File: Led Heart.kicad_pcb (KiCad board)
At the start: 2 copper layers, 32.2 x 28.7 mm, 38 parts, among them J1 Conn_01x03_Female, J2 Conn_01x02_Female, SW1 SW_DIP_x01, U1 STM32L031G6U6

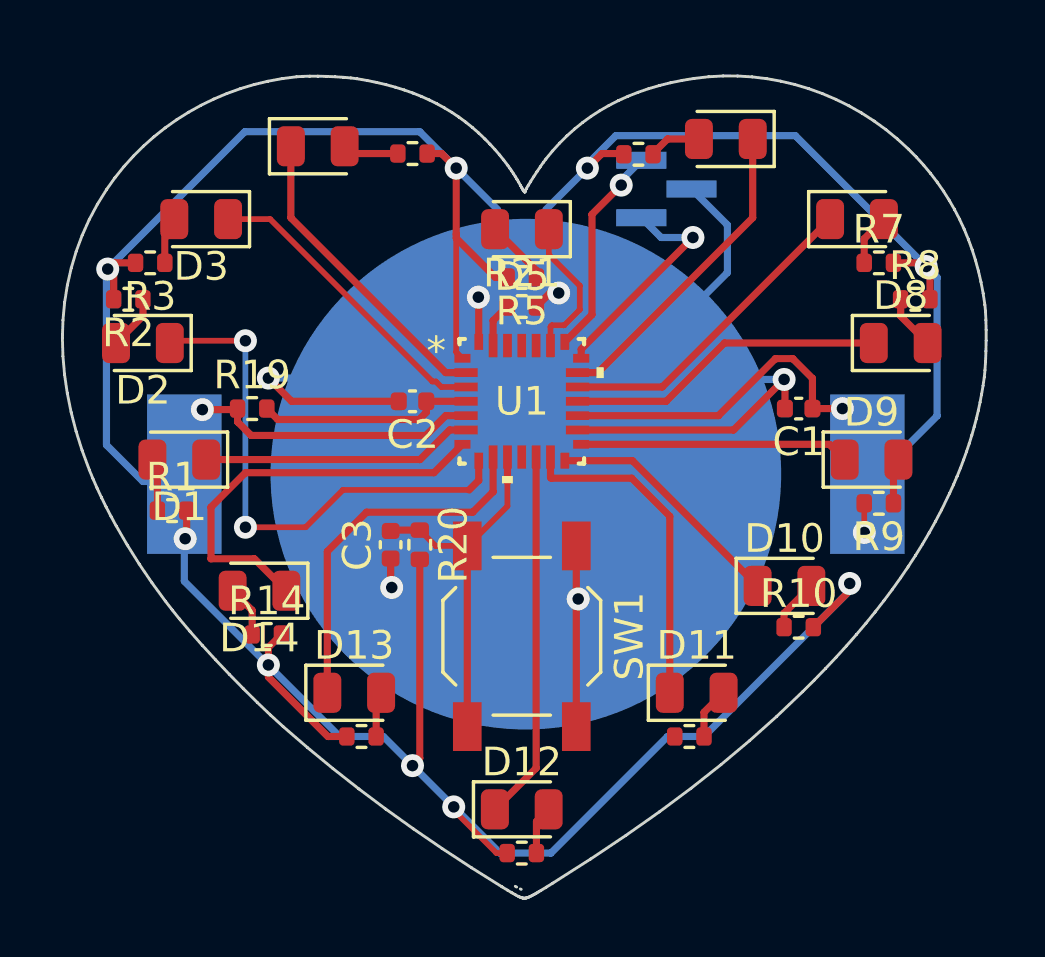
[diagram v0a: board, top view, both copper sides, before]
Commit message: Usuniety projekt emila dodany przypadkiem i ostatnie chyba poprawki
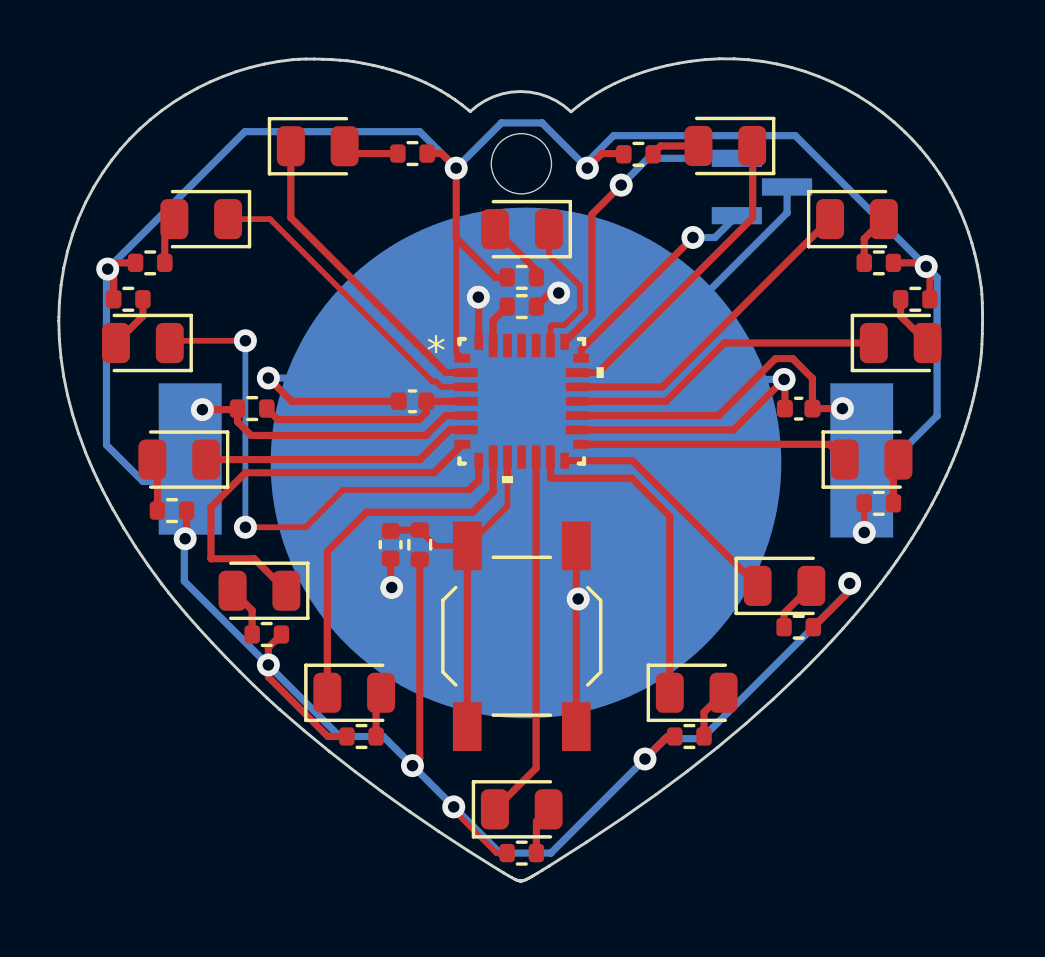
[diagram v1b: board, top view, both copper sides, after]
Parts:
- added REF**: MountingHole_2.1mm, MountingHole:MountingHole_2.1mm, F.Cu at (106.9, 84.4)
- J2: footprint Battery:BatteryHolder_MPD_BC2003_1x2032 -> SamacSys_Parts:BatteryHolder_MPD_BC2003_1x2032
- moved J1 3.33 mm to (115.3, 85.2)
- moved J2 0.39 mm to (107.1, 94.9)
- moved D6 0.24 mm to (114.0, 83.8)
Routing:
- net Net-(J1-Pad3): track 7.43 -> 10.7 mm
- net +3V0: track 143.3 -> 146.5 mm, vias 12 -> 13
- net GND: track 65.5 -> 67.4 mm
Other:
- outline, holes or cut-outs redrawn

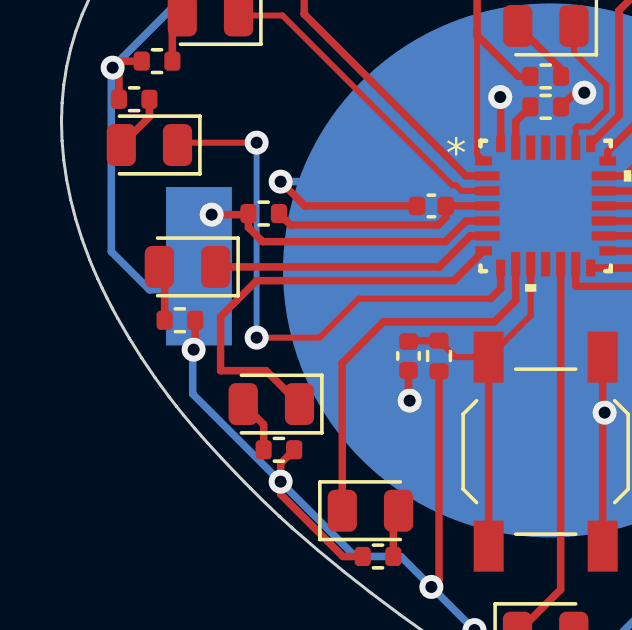
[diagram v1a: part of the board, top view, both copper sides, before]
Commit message: okkk
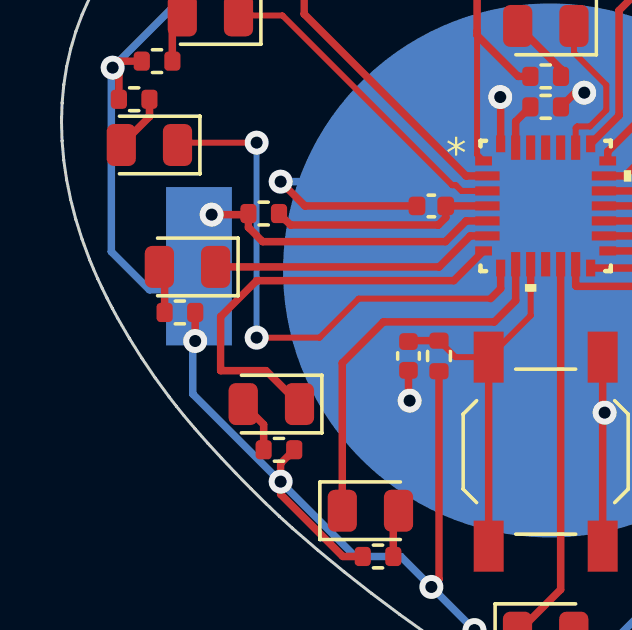
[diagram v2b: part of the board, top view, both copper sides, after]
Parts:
- moved R1 0.26 mm to (94.7, 96.3)
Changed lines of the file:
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@@
   )
   (footprint "Resistor_SMD:R_0402_1005Metric" (layer "F.Cu")
-    (at 94.742 96.52)
+    (at 94.742 96.26)
     (descr "Resistor SMD 0402 (1005 Metric), square (rectangular) end terminal, IPC_7351 nominal, (Body size source: IPC-SM-782 page 72, https://www.pcb-3d.com/wordpress/wp-content/uploads/ipc-sm-782a_amendment_1_and_2.pdf), generated with kicad-footprint-generator")
     (tags "resistor")
@@
   (gr_line (start 98.953544 80.800999) (end 99.161225 80.786298) (layer "Edge.Cuts") (width 0.1))
   (segment (start 94.232 94.9155) (end 94.0585 94.742) (width 0.25) (layer "F.Cu") (net 1))
-  (segment (start 94.232 96.52) (end 94.232 94.9155) (width 0.25) (layer "F.Cu") (net 1))
+  (segment (start 94.232 96.26) (end 94.232 94.9155) (width 0.25) (layer "F.Cu") (net 1))
   (segment (start 93.728 89.7385) (end 92.7885 90.678) (width 0.25) (layer "F.Cu") (net 2))
   (segment (start 93.728 89.154) (end 93.728 89.7385) (width 0.25) (layer "F.Cu") (net 2))
@@
   (segment (start 104.562 106.968479) (end 106.051521 108.458) (width 0.2) (layer "F.Cu") (net 16))
   (segment (start 109.728 84.074) (end 109.22 84.582) (width 0.25) (layer "F.Cu") (net 16))
+  (segment (start 95.252 97.212) (end 95.252 96.26) (width 0.25) (layer "F.Cu") (net 16))
   (segment (start 103.634 84.074) (end 104.14 84.074) (width 0.25) (layer "F.Cu") (net 16))
   (segment (start 96.99 93) (end 97.026 92.964) (width 0.25) (layer "F.Cu") (net 16))
@@
   (segment (start 97.5 93.9) (end 97.026 93.426) (width 0.25) (layer "F.Cu") (net 16))
   (segment (start 110.488 84.074) (end 109.728 84.074) (width 0.25) (layer "F.Cu") (net 16))
-  (segment (start 95.252 97.448) (end 95.2 97.5) (width 0.25) (layer "F.Cu") (net 16))
   (segment (start 104.9909 93.209999) (end 104.282102 93.209999) (width 0.25) (layer "F.Cu") (net 16))
   (segment (start 104.648 86.888) (end 104.648 90.9941) (width 0.2) (layer "F.Cu") (net 16))
@@
   (segment (start 118.872 97.282) (end 118.872 96.268) (width 0.2) (layer "F.Cu") (net 16))
   (segment (start 104.648 86.888) (end 104.648 87.023834) (width 0.25) (layer "F.Cu") (net 16))
-  (segment (start 95.252 96.52) (end 95.252 97.448) (width 0.25) (layer "F.Cu") (net 16))
   (segment (start 98.1 101.9) (end 98.1 101.292) (width 0.25) (layer "F.Cu") (net 16))
   (segment (start 92.716 87.884) (end 92.5 88.1) (width 0.25) (layer "F.Cu") (net 16))
@@
   (via (at 118.11 92.964) (size 0.8) (drill 0.4) (layers "F.Cu" "B.Cu") (net 16))
   (via (at 104.648 84.582) (size 0.8) (drill 0.4) (layers "F.Cu" "B.Cu") (net 16))
-  (via (at 95.2 97.5) (size 0.8) (drill 0.4) (layers "F.Cu" "B.Cu") (net 16))
+  (via (at 95.252 97.212) (size 0.8) (drill 0.4) (layers "F.Cu" "B.Cu") (net 16))
   (via (at 118.872 97.282) (size 0.8) (drill 0.4) (layers "F.Cu" "B.Cu") (net 16))
   (segment (start 104.648 84.582) (end 106.225001 83.004999) (width 0.25) (layer "B.Cu") (net 16))
